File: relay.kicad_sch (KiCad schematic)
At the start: 5 parts, among them J3 Screw_Terminal_01x04, K2 G2RL-2, Q1 BC547

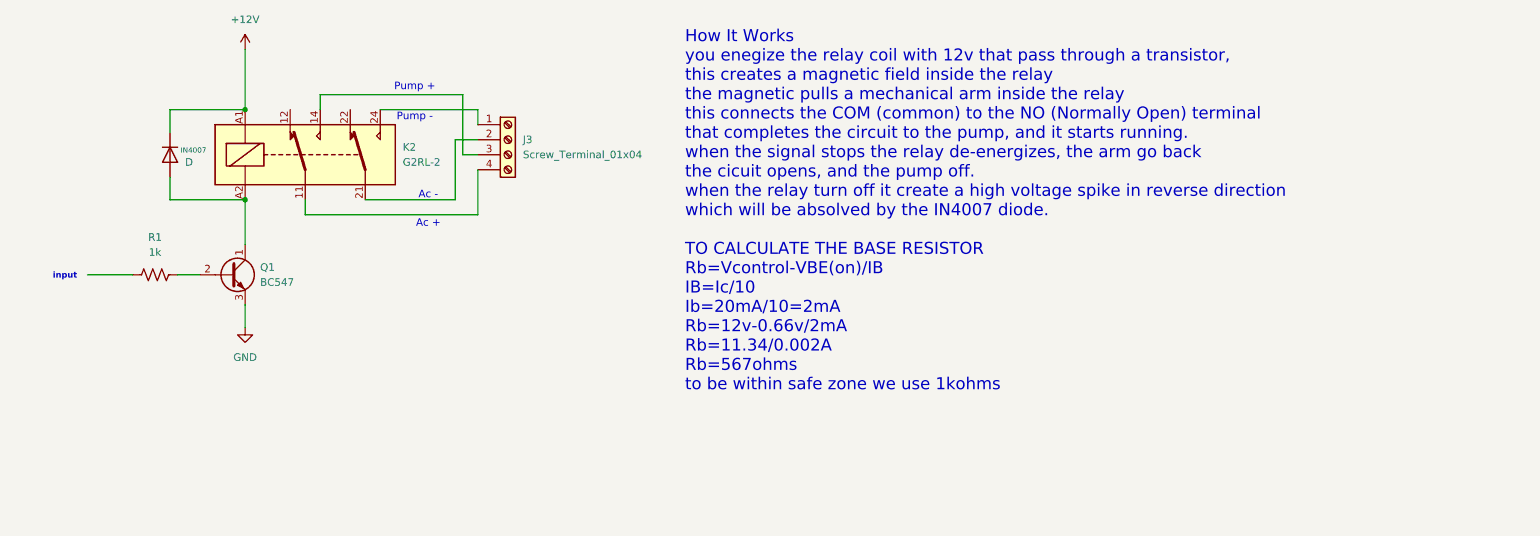
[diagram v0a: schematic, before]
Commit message: relay subsheet
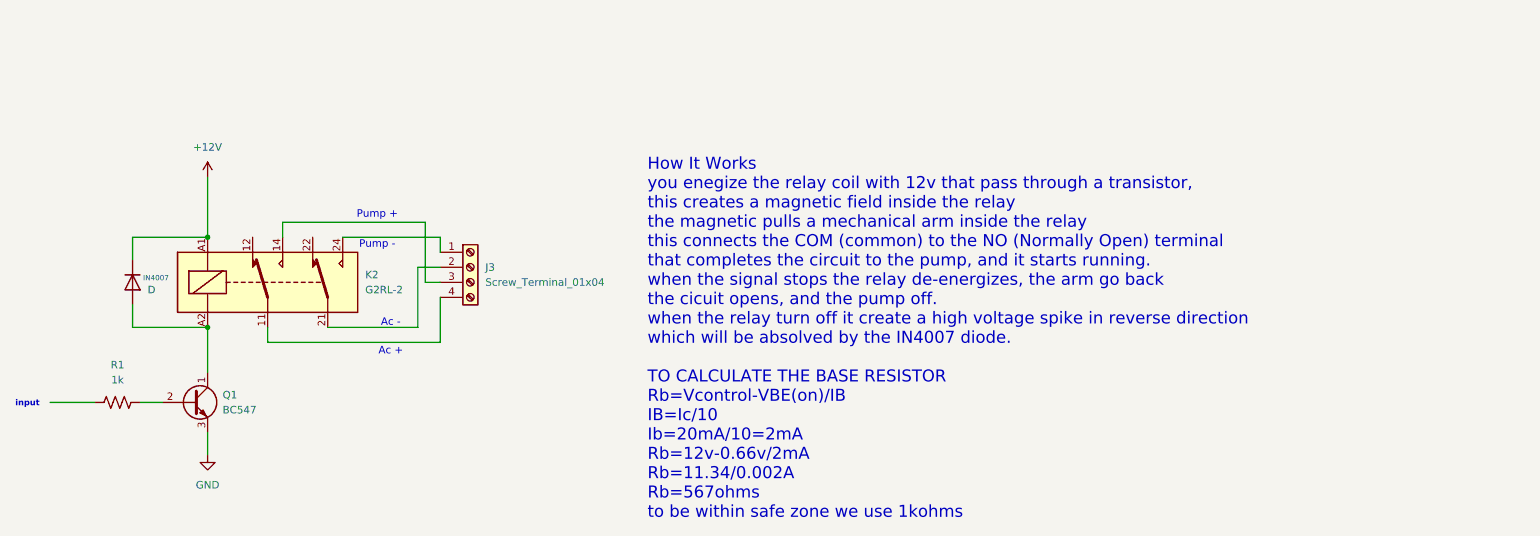
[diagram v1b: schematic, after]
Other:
- moved on the sheet: IN4007, J3, K2, Q1, R1
